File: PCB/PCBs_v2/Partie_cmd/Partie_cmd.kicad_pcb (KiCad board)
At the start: 4 copper layers, 67 parts, among them J10 Conn_01x02, J2 Conn_01x04_Socket, J3 Conn_01x04_Socket, J6 Conn_01x04, J7 Conn_01x04, J9 Conn_01x02, U1 ESP32-S3-DEVKITC-1-N8R2, U2 BU18SD5WG-TL, U3 BU33SD5WG-TR, U4 XL1509-5.0

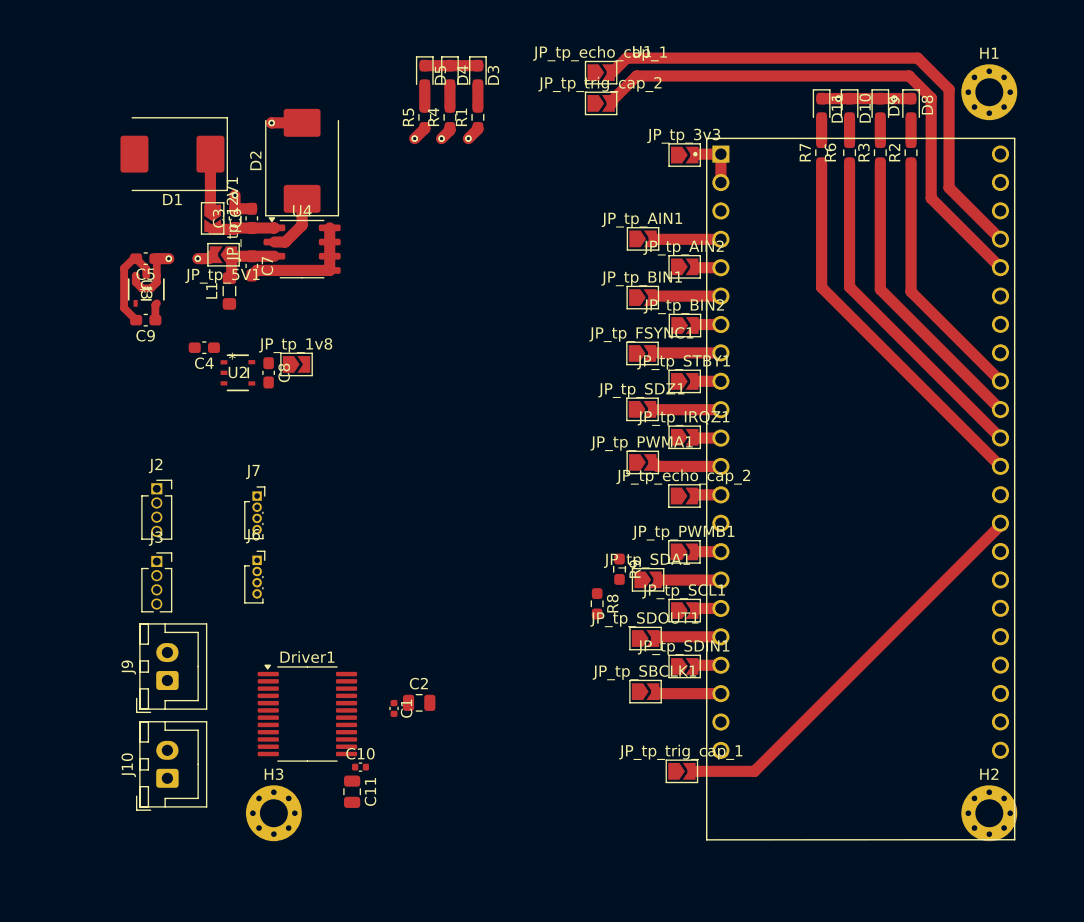
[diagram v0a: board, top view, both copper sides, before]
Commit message: Routage pcb cmd
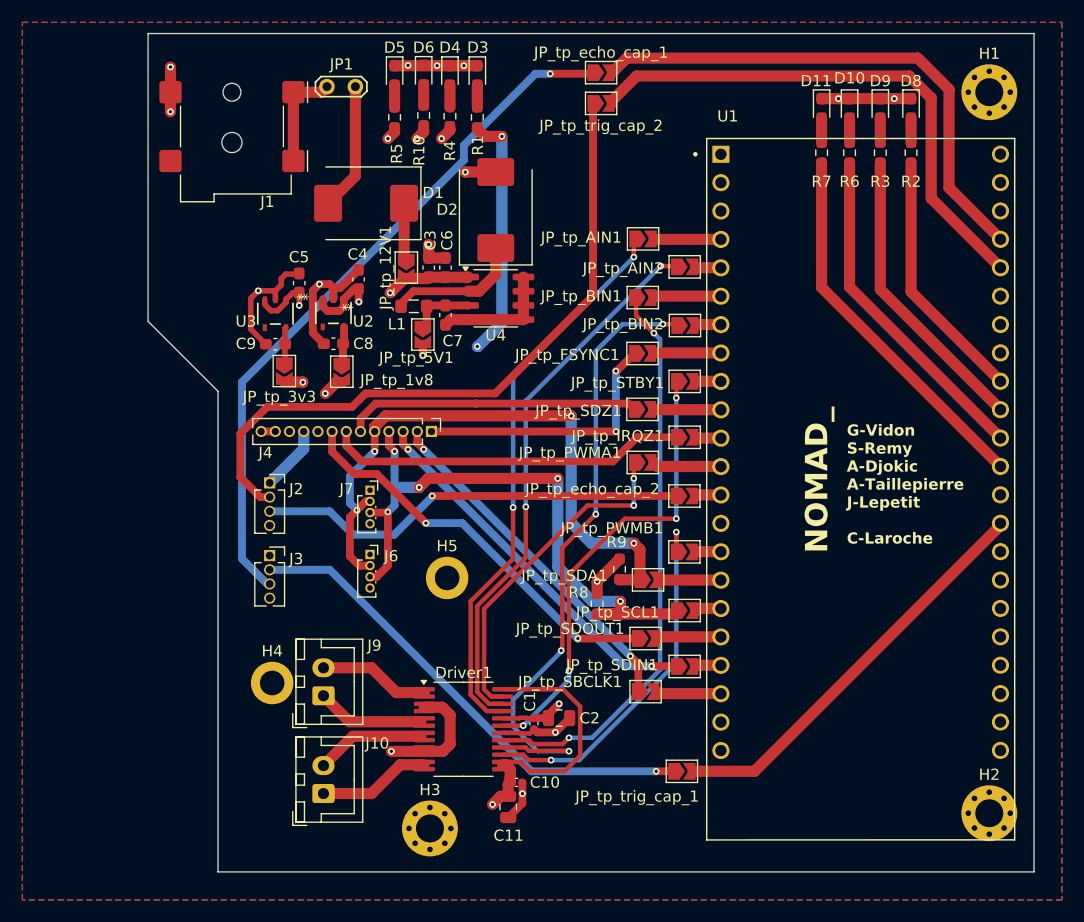
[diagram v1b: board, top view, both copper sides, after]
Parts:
- added D6: LED_Small, LED_SMD:LED_0603_1608Metric_Pad1.05x0.95mm_HandSolder, F.Cu at (130.4, 48.7)
- added H4: MountingHole_Pad, MountingHole:MountingHole_2.2mm_M2_DIN965_Pad, F.Cu at (116.8, 103.1)
- added H5: MountingHole_Pad, MountingHole:MountingHole_2.2mm_M2_DIN965_Pad, F.Cu at (132.5, 93.7)
- added J1: Barrel_Jack, Connector_BarrelJack:BarrelJack_Wuerth_694108106102_2.5x5.5mm, F.Cu at (113.2, 53.3)
- added J4: Conn_01x13_Pin, Connector_PinHeader_1.27mm:PinHeader_1x13_P1.27mm_Vertical, F.Cu at (131.1, 80.6)
- added JP1: Jumper_2_Bridged, TestPoint:TestPoint_2Pads_Pitch2.54mm_Drill0.8mm, F.Cu at (121.8, 49.8)
- added R10: 1.2k, Resistor_SMD:R_0603_1608Metric_Pad0.98x0.95mm_HandSolder, F.Cu at (130.4, 52.3)
- R4: value 120 -> 1.2k
- R5: value 82 -> 820
- moved JP_tp_3v3 40.7 mm to (117.9, 75.2), turned to -90 degrees
- moved JP_tp_5V1 19.2 mm to (130.3, 71.9), turned to -90 degrees
- moved D1 17.9 mm to (125.2, 60.2)
- moved C3 17.9 mm to (130.8, 65.9)
- moved C6 17.9 mm to (132.3, 65.9)
- moved C7 17.9 mm to (132.3, 70.2)
- moved D2 17.9 mm to (136.8, 60.8)
- moved JP_tp_12V1 17.9 mm to (128.8, 65.9)
- moved U4 17.9 mm to (136.8, 68.7)
- moved L1 16.6 mm to (129.5, 69.4), turned to 0 degrees
- moved C4 15.1 mm to (124.6, 67.0), turned to 90 degrees
- moved C10 14.0 mm to (138.7, 112.0)
- moved C11 14.0 mm to (138.0, 114.2)
- moved Driver1 14.0 mm to (134.0, 107.2)
- moved H3 14.0 mm to (131.0, 116.1)
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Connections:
- C1 pad 1: 5V -> 3.3V
- C2 pad 1: 5V -> 3.3V
- Driver1 pad 20: 5V -> 3.3V
- Driver1 pad 3: (no net) -> GND
- R4 pad 1: 3.3V -> 5V
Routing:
- net 12V: track 6.92 -> 184.8 mm, vias 1 -> 4
- net 5V: track 7.77 -> 168.9 mm, vias 2 -> 5
- net 3.3V: track 6.13 -> 118.0 mm, vias 1 -> 3
- net Echo_cap_1: track 0.00 -> 62.9 mm, vias 0 -> 1
- net Trig_cap_2: track 0.00 -> 61.1 mm
- net BIN2: track 0.00 -> 56.9 mm, vias 0 -> 4
- net SCL: track 0.00 -> 56.3 mm, vias 0 -> 5
- net SDA: track 0.00 -> 55.9 mm, vias 0 -> 4
- net BIN1: track 0.00 -> 51.2 mm, vias 0 -> 2
- net AIN1: track 0.00 -> 50.3 mm, vias 0 -> 2
- net AIN2: track 0.00 -> 49.1 mm, vias 0 -> 2
- net GND: track 37.6 -> 86.3 mm, vias 4 -> 14
- net Trig_cap_1: track 0.00 -> 43.6 mm, vias 0 -> 1
- net STBY: track 0.00 -> 41.0 mm, vias 0 -> 4
- net 1.8V: track 1.36 -> 41.7 mm, vias 1 -> 2
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- added copper zone on In1.Cu, net 1.8V
- added copper zone on In1.Cu, net 12V
- added copper zone on In1.Cu, net 3.3V
- added copper zone on In1.Cu, net 5V
- added copper zone on B.Cu, net GND
- added copper zone on F.Cu, net GND
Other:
- board outline added: 79.2 x 75 mm
- board text added: "G-Vidon S-Remy A-Djokic A-Taillepierre J-Lepetit C-Laroche"
- board text added: "NOMAD_"
